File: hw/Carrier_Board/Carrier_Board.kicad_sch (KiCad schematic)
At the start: 20 parts, among them J1 Conn_01x05

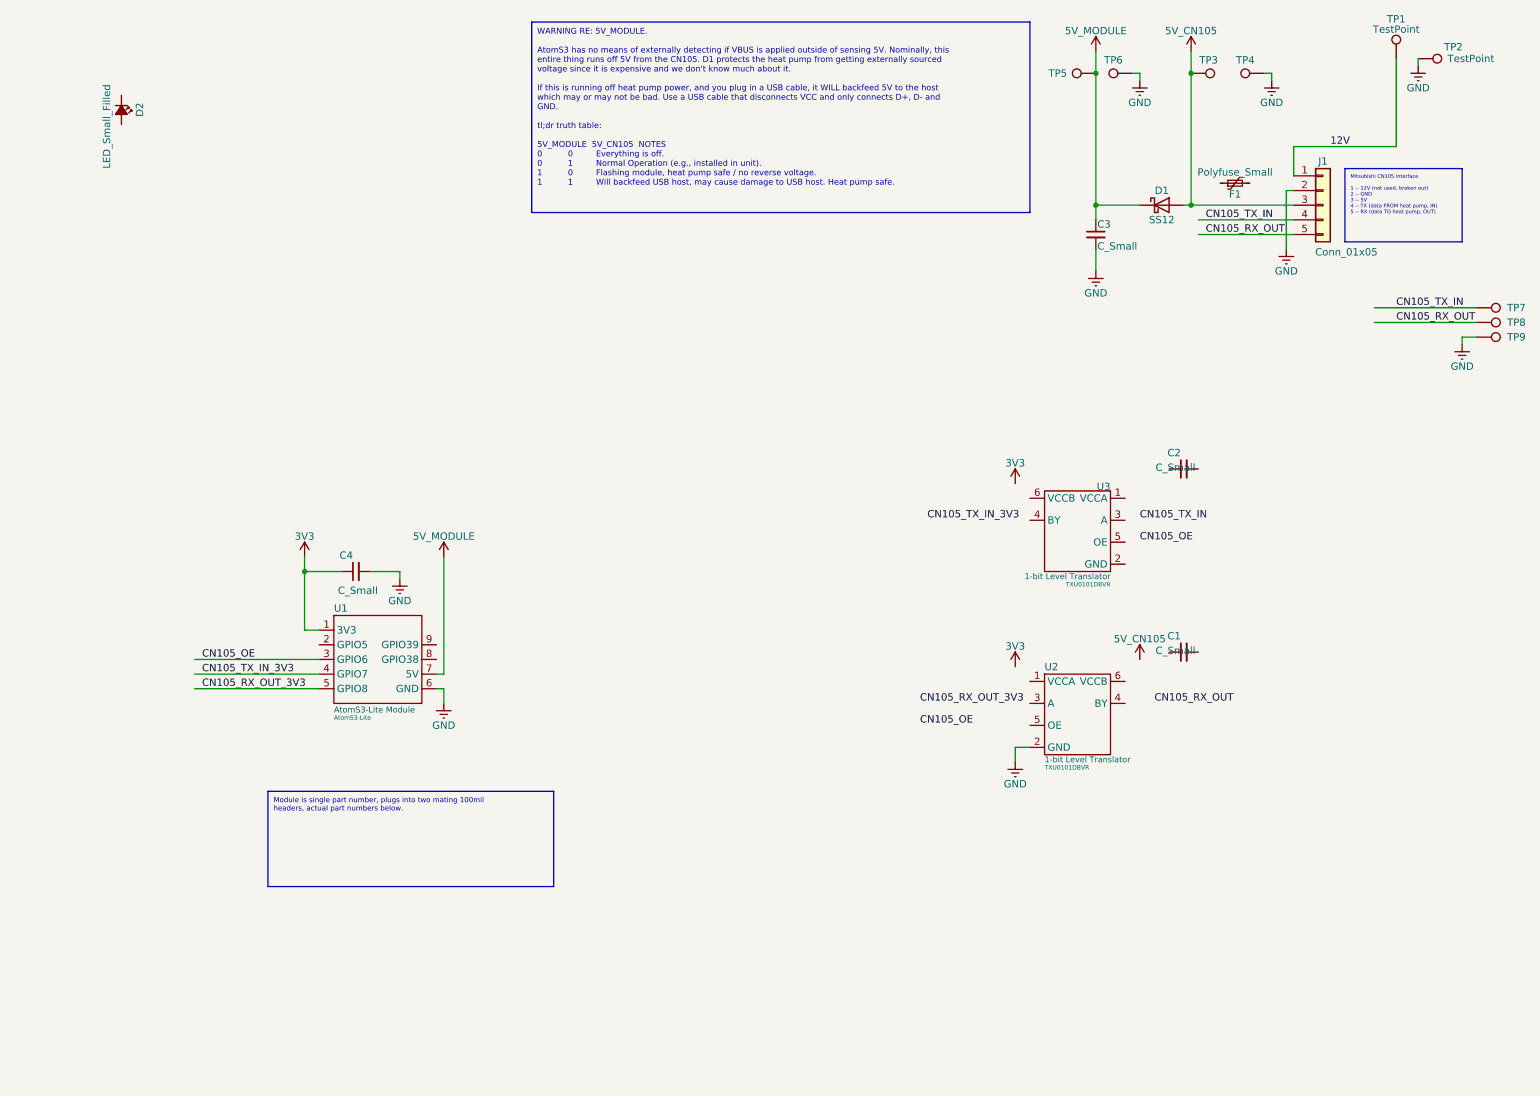
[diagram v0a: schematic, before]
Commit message: hw: initial schematic mostly done, pushing for reference
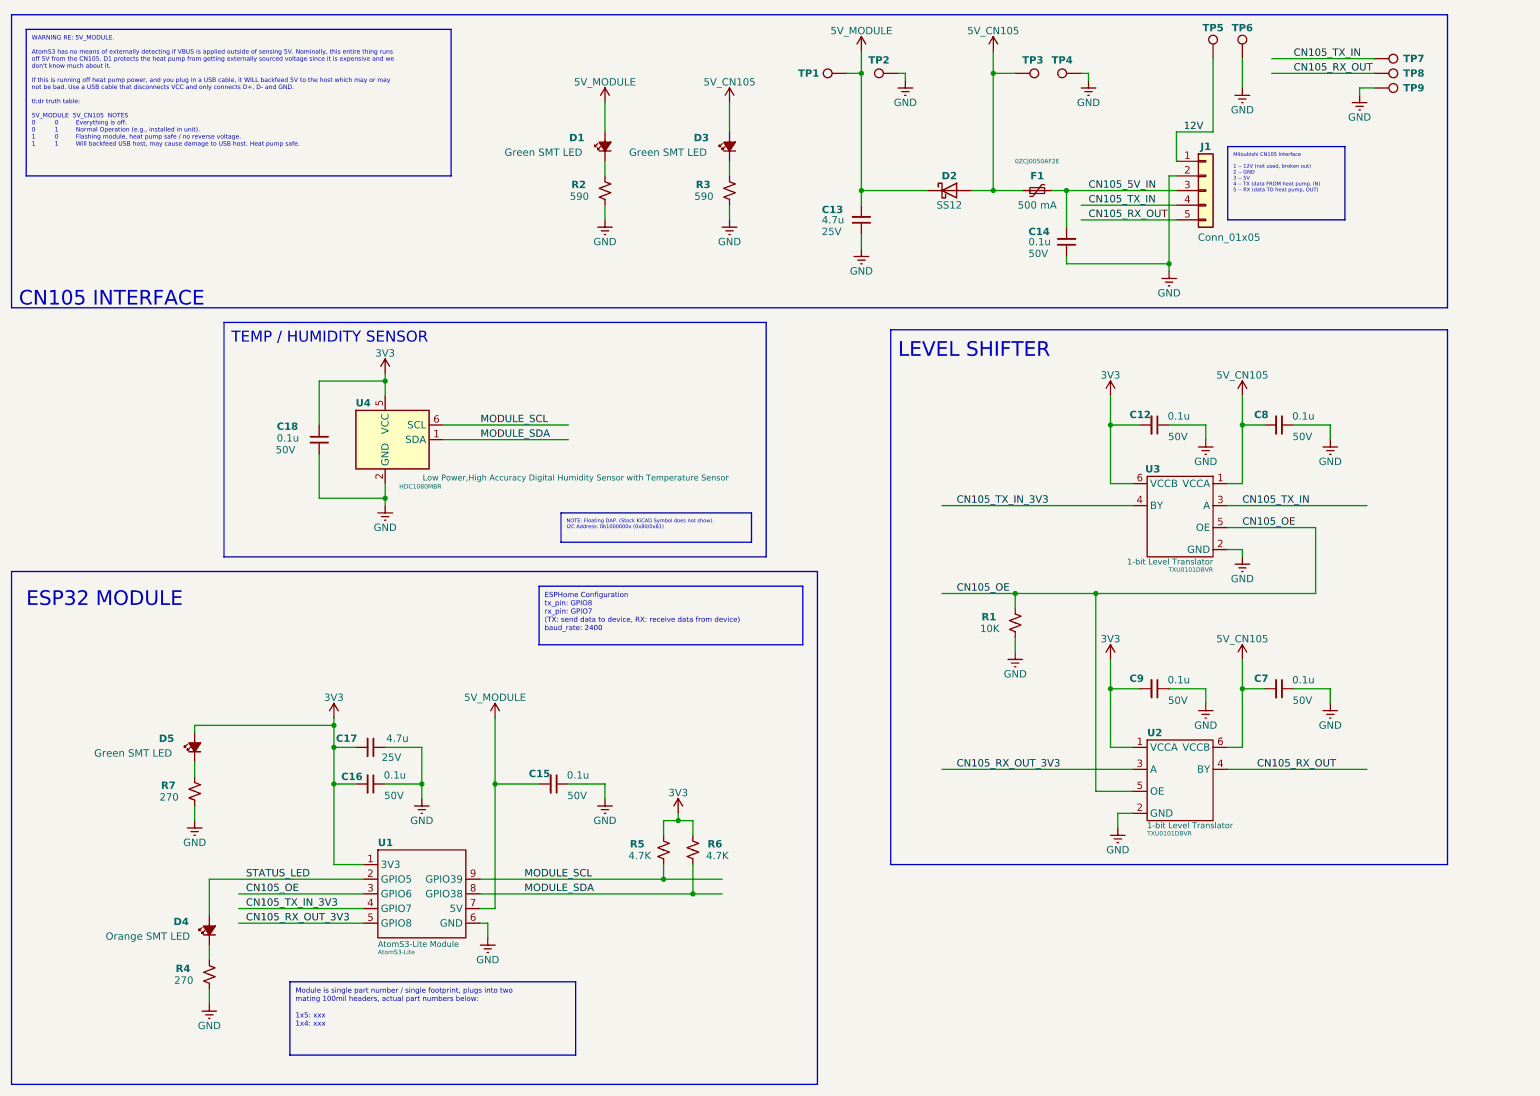
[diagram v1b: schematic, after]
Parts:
- removed C1, C2, C3, C4: C_Small, symbol Device:C_Small
- added C12, C14, C15, C16, C18, C7, C8, C9: 0.1u, Capacitor_SMD:C_0603_1608Metric_Pad1.08x0.95mm_HandSolder, symbol Device:C_Small
- added C13, C17: 4.7u, Capacitor_SMD:C_0805_2012Metric_Pad1.18x1.45mm_HandSolder, symbol Device:C_Small
- added D3, D4, D5: LED_Small_Filled, LED_SMD:LED_0603_1608Metric_Pad1.05x0.95mm_HandSolder, symbol Device:LED_Small_Filled
- added R1: 10K, Resistor_SMD:R_0603_1608Metric_Pad0.98x0.95mm_HandSolder, symbol Device:R_Small_US
- added R2, R3: 590, Resistor_SMD:R_0603_1608Metric_Pad0.98x0.95mm_HandSolder, symbol Device:R_Small_US
- added R4, R7: 270, Resistor_SMD:R_0603_1608Metric_Pad0.98x0.95mm_HandSolder, symbol Device:R_Small_US
- added R5, R6: 4.7K, Resistor_SMD:R_0603_1608Metric_Pad0.98x0.95mm_HandSolder, symbol Device:R_Small_US
- added U4: HDC1080, Package_SON:Texas_PWSON-N6, symbol Sensor_Humidity:HDC1080
- D1: renamed from D2; footprint (none) -> LED_SMD:LED_0603_1608Metric_Pad1.05x0.95mm_HandSolder; Comment (none) -> Green SMT LED
- F1: value Polyfuse_Small -> 500 mA; footprint (none) -> Fuse:Fuse_1206_3216Metric_Pad1.42x1.75mm_HandSolder; ManufacturerPartNumber (none) -> 0ZCJ0050AF2E
- TP1: renamed from TP5; footprint (none) -> TestPoint:TestPoint_Keystone_5005-5009_Compact
- TP2: renamed from TP6; footprint (none) -> TestPoint:TestPoint_Keystone_5005-5009_Compact
- TP3, TP4, TP7, TP8, TP9: footprint (none) -> TestPoint:TestPoint_Keystone_5005-5009_Compact
- TP5: renamed from TP1; footprint (none) -> TestPoint:TestPoint_Keystone_5005-5009_Compact
- TP6: renamed from TP2; footprint (none) -> TestPoint:TestPoint_Keystone_5005-5009_Compact
- renumbered D1 to D2
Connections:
- net 3V3: now also U2.1 (VCCA), U3.6 (VCCB), C12.2, C16.2, C17.2, C18.1, C9.2, D5.2 (A), R5.1, R6.1, U4.5 (VCC)
- net 5V_CN105: now also F1.1, U2.6 (VCCB), U3.1 (VCCA), C7.2, C8.2, D3.2 (A); no longer J1.3 (Pin_3)
- net 5V_MODULE: now also D1.2 (A), C13.2, C15.2
- net CN105_OE: now also U2.5 (OE), U3.5 (OE), R1.1
- net CN105_RX_OUT: now also U2.4 (BY)
- net CN105_RX_OUT_3V3: now also U2.3 (A)
- net CN105_TX_IN: now also U3.3 (A)
- net CN105_TX_IN_3V3: now also U3.4 (BY)
- net GND: now also U3.2 (GND), C12.1, C13.1, C14.1, C15.1, C16.1, C17.1, C18.2, C7.1, C8.1, C9.1, R1.2, R2.2, R3.2, R4.2, R7.2, U4.2 (GND)
- net CN105_5V_IN: now reaches F1.2
- net CN105_5V_IN: now also J1.3 (Pin_3), C14.2
- net at D1.1 (K): now also R2.1
- net STATUS_LED: now reaches U1.2 (GPIO5)
- net STATUS_LED: now also D4.2 (A)
- net MODULE_SDA: now reaches U1.8 (GPIO38)
- net MODULE_SDA: now also R6.2, U4.1 (SDA)
- net MODULE_SCL: now reaches U1.9 (GPIO39)
- net MODULE_SCL: now also R5.2, U4.6 (SCL)
- new net: D5.1 (K), R7.1
- new net: D3.1 (K), R3.1
- new net: D4.1 (K), R4.1
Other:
- note added: "CN105 INTERFACE"
- note added: "ESP32 MODULE"
- note added: "LEVEL SHIFTER"
- note added: "TEMP / HUMIDITY SENSOR"
- title: (none) -> CN105 Interface Board
- moved on the sheet: D1, D2, F1, J1, TP1, TP2, TP3, TP4, TP5, TP6, TP7, TP8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
